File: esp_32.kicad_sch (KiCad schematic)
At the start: 20 parts, among them J1 USB_B_Micro, J2 Conn_01x22_Pin, U1 ESP32-S3-MINI-1, U2 D3V3XA4B10LP, U3 TLV75801PDRV, U4 ENS210

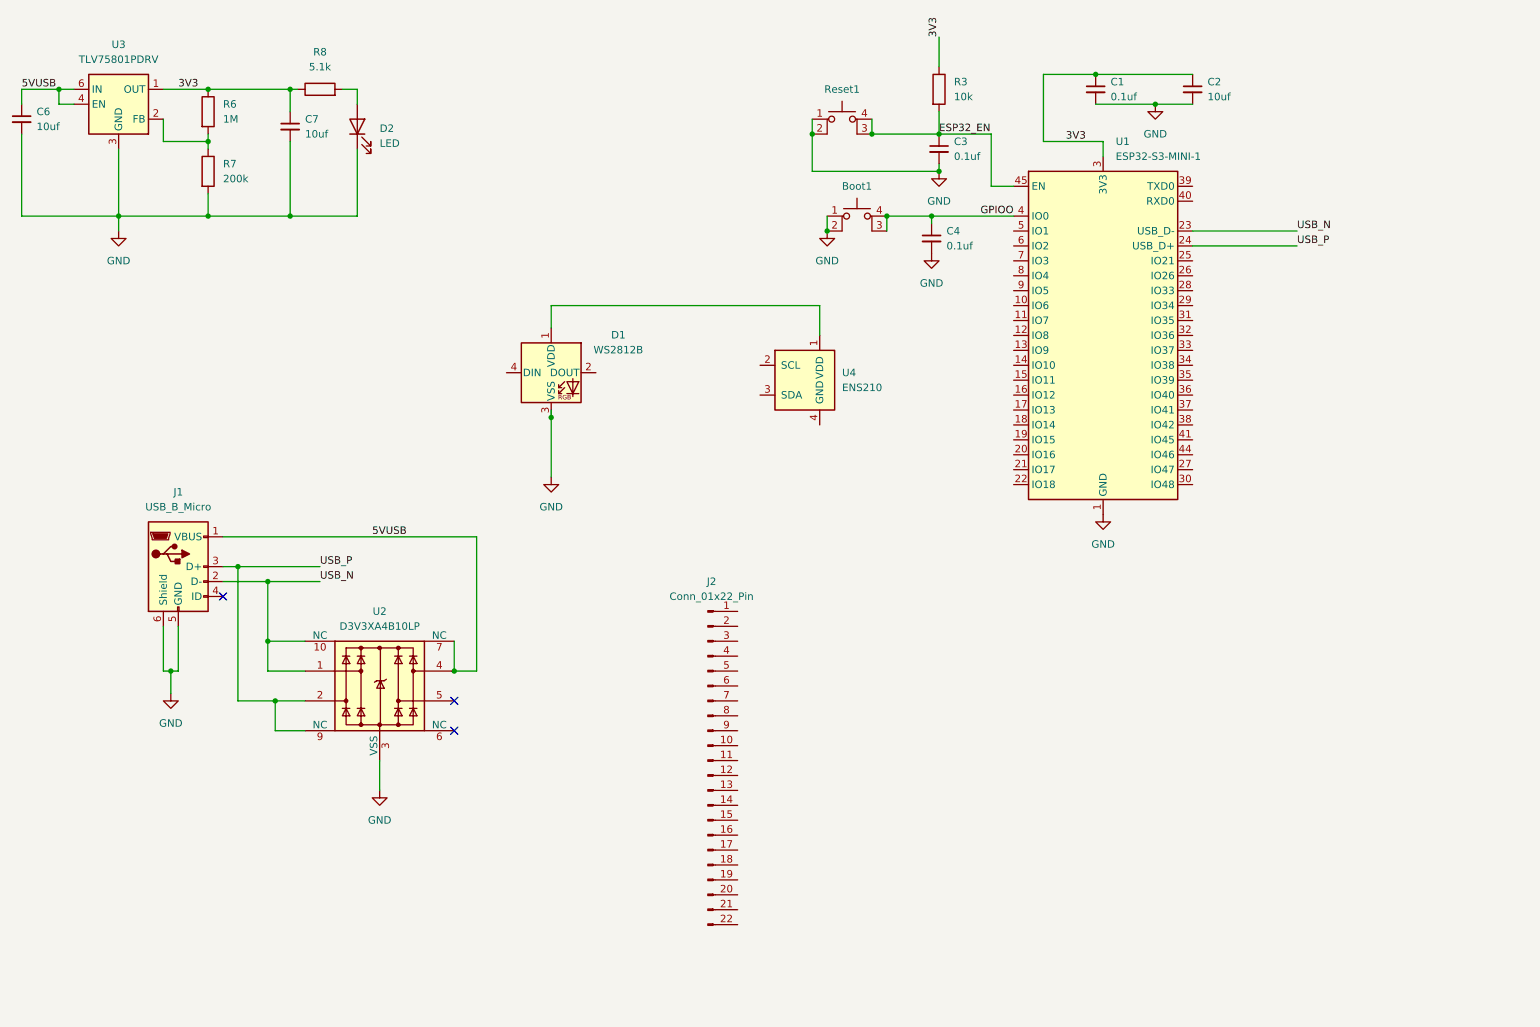
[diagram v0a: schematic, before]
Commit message: schematic
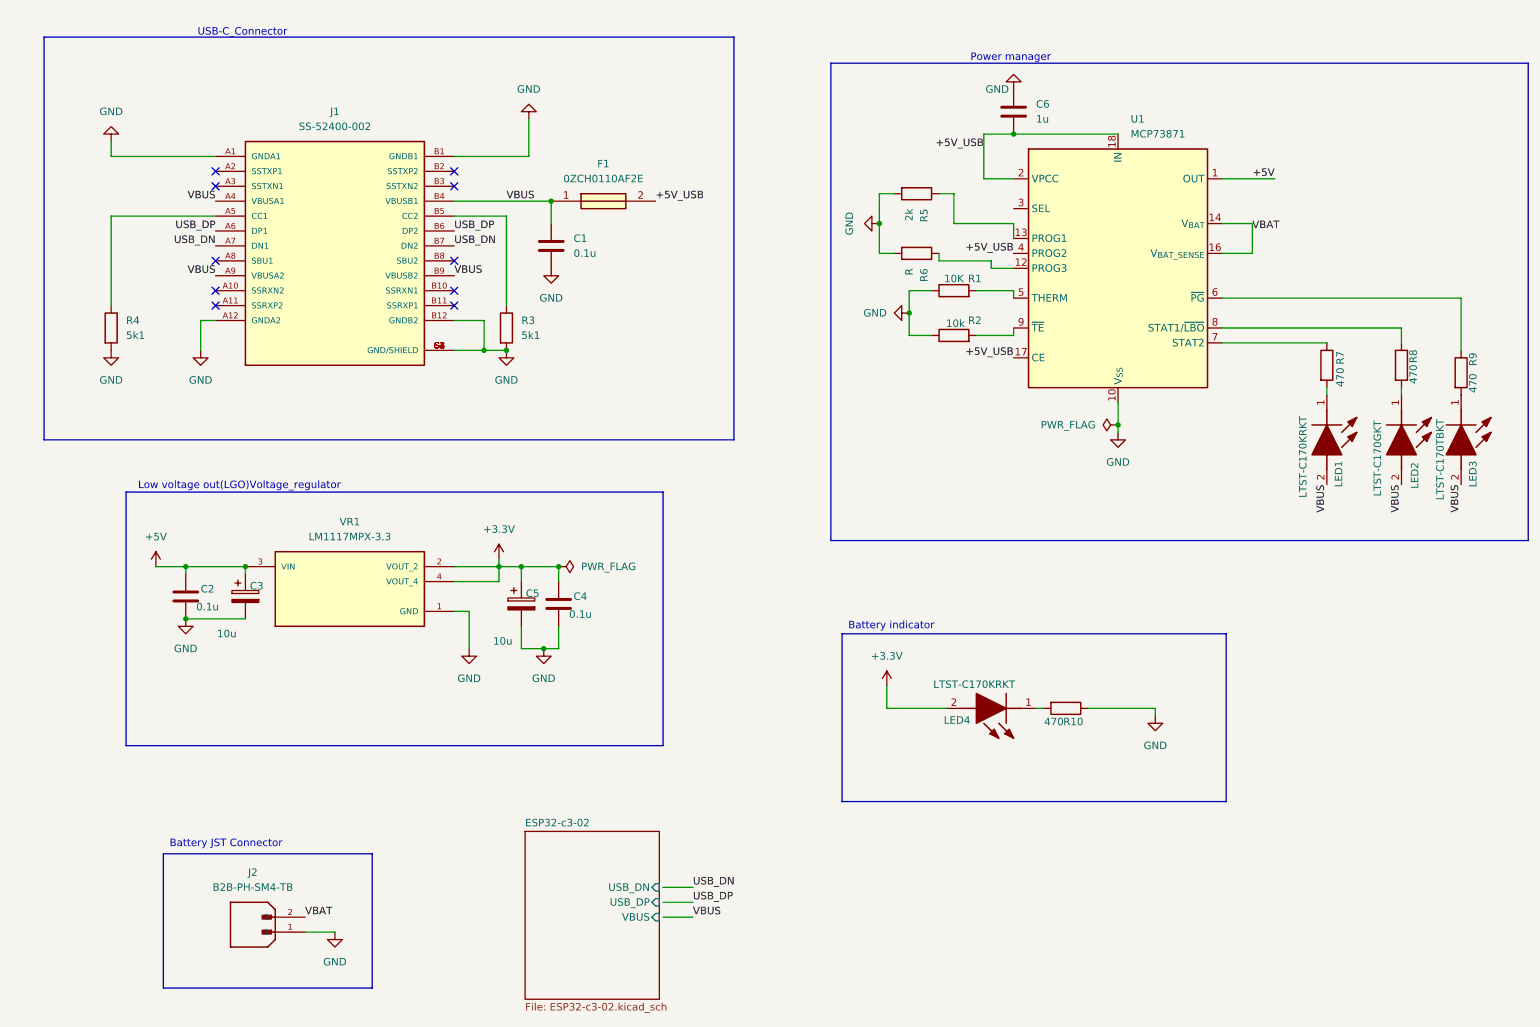
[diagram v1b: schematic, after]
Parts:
- removed Boot1, Reset1: SW_MEC_5E, Button_Switch_SMD:SW_DIP_SPSTx02_Slide_6.7x6.64mm_W6.73mm_P2.54mm_LowProfile_JPin, symbol Switch:SW_MEC_5E
- removed C1, C4: 0.1uf, Capacitor_SMD:C_0603_1608Metric, symbol Device:C_Small
- removed C2, C6, C7: 10uf, Capacitor_SMD:C_0603_1608Metric, symbol Device:C_Small
- removed C3: 0.1uf, Connector_Samtec_HPM_THT:Samtec_HPM-08-01-x-S_Straight_1x08_Pitch5.08mm, symbol Device:C_Small
- removed D1: WS2812B, LED_SMD:LED_WS2812B_PLCC4_5.0x5.0mm_P3.2mm, symbol LED:WS2812B
- removed D2: LED, LED_SMD:LED_0603_1608Metric, symbol Device:LED
- removed J1: USB_B_Micro, Connector_USB:USB_Micro-B_Molex-105017-0001, symbol Connector:USB_B_Micro
- removed J2: Conn_01x22_Pin, Connector_PinSocket_1.27mm:PinSocket_1x22_P1.27mm_Vertical, symbol Connector:Conn_01x22_Pin
- removed U1: ESP32-S3-MINI-1, RF_Module:ESP32-S2-MINI-1, symbol RF_Module:ESP32-S3-MINI-1
- removed U2: D3V3XA4B10LP, Package_DFN_QFN:Diodes_UDFN-10_1.0x2.5mm_P0.5mm, symbol Power_Protection:D3V3XA4B10LP
- removed U3: TLV75801PDRV, Package_SON:WSON-6-1EP_2x2mm_P0.65mm_EP1x1.6mm, symbol Regulator_Linear:TLV75801PDRV
- removed U4: ENS210, Package_DFN_QFN:AMS_QFN-4-1EP_2x2mm_P0.95mm_EP0.7x1.6mm, symbol Sensor_Humidity:ENS210
- added C1, C2, C4: 0.1u, symbol Device:C
- added C3, C5: 10u, symbol Device:C_Polarized
- added C6: 1u, symbol Device:C
- added F1: 0ZCH0110AF2E, FUSC3226X100N, symbol 0ZCH0110AF2E:0ZCH0110AF2E
- added J1: SS-52400-002, SS-52400-002:BELFUSE_SS-52400-002, symbol SS-52400-002:SS-52400-002
- added J2: B2B-PH-SM4-TB, B2B-PH-SM4-TB:JST_B2B-PH-SM4-TB, symbol B2B-PH-SM4-TB:B2B-PH-SM4-TB
- added LED1, LED4: LTST-C170KRKT, LEDC2012X120N, symbol LTST-C170KRKT:LTST-C170KRKT
- added LED2: LTST-C170GKT, LEDC2012X120N, symbol LTST-C170GKT:LTST-C170GKT
- added LED3: LTST-C170TBKT, LEDC2012X120N, symbol LTST-C170TBKT:LTST-C170TBKT
- added R1: 10K, symbol Device:R
- added R10, R9: 470, symbol Device:R
- added R2: 10k, symbol Device:R
- added R4: 5k1, symbol Device:R
- added R5: 2k, symbol Device:R
- added U1: MCP73871, Package_DFN_QFN:QFN-20-1EP_4x4mm_P0.5mm_EP2.5x2.5mm, symbol Battery_Management:MCP73871
- added VR1: LM1117MPX-3.3, LM1117MPX-3.3:VREG_LM1117MPX-3.3, symbol LM1117MPX-3.3:LM1117MPX-3.3
- R3: value 10k -> 5k1; footprint Resistor_SMD:R_0603_1608Metric -> (none)
- R6: value 1M -> R; footprint Resistor_SMD:R_0603_1608Metric -> (none)
- R7: value 200k -> 470; footprint Resistor_SMD:R_0603_1608Metric -> (none)
- R8: value 5.1k -> 470; footprint Resistor_SMD:R_0603_1608Metric -> (none)
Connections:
- net ESP32_EN is gone; now on net GND: R3.2
- net GND: now also R6.2, C1.2, C2.2, C3.2, C4.2, C5.2, C6.1, J1.A1 (GNDA1), J1.A12 (GNDA2), J1.B1 (GNDB1), J1.B12 (GNDB2), J1.G1 (GND/SHIELD), J1.G2 (GND/SHIELD), J1.G3 (GND/SHIELD), J1.G4 (GND/SHIELD), J1.S1 (GND/SHIELD), J1.S2 (GND/SHIELD), J1.S3 (GND/SHIELD), J1.S4 (GND/SHIELD), J2.1, R1.1, R10.1, R2.1, R4.2, R5.2, U1.10 (V_{SS}), U1.11 (V_{SS}), U1.21 (V_{SS}), VR1.1 (GND); no longer R7.2
- net at R7.1: now also U1.7 (STAT2); no longer R6.2
- net at R8.2: now also LED2.1 (K)
- removed net 3V3: R3.1, R6.1, R8.1
- new net: R6.1, U1.12 (PROG3)
- new net: R5.1, U1.13 (PROG1)
- new net: R1.2, U1.5 (THERM)
- new net: R9.1, U1.6 (~{PG})
- new net: R8.1, U1.8 (STAT1/~{LBO})
- new net: R2.2, U1.9 (~{TE})
- new net: LED1.1 (K), R7.2
- new net: J1.A5 (CC1), R4.1
- new net: J1.B5 (CC2), R3.1
- new net: LED3.1 (K), R9.2
- new net: LED4.1 (K), R10.2
- new net +3.3V: C4.1, C5.1, LED4.2 (A), VR1.2 (VOUT_2), VR1.4 (VOUT_4)
- new net +5V: C2.1, C3.1, U1.1 (OUT), U1.20 (OUT), VR1.3 (VIN)
- new net +5V_USB: C6.2, F1.2, U1.17 (CE), U1.18 (IN), U1.19 (IN), U1.2 (VPCC), U1.4 (PROG2)
- new net USB_DN: J1.A7 (DN1), J1.B7 (DN2)
- new net USB_DP: J1.A6 (DP1), J1.B6 (DP2)
- new net VBAT: J2.2, U1.14 (V_{BAT}), U1.15 (V_{BAT}), U1.16 (V_{BAT_SENSE})
- new net VBUS: C1.1, F1.1, J1.A4 (VBUSA1), J1.A9 (VBUSA2), J1.B4 (VBUSB1), J1.B9 (VBUSB2), LED1.2 (A), LED2.2 (A), LED3.2 (A)
- no-connect marks 3 -> 10
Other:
- added sheet ESP32-c3-02 (ESP32-c3-02.kicad_sch)
- note added: "Battery JST Connector"
- note added: "Battery indicator"
- note added: "Low voltage out(LGO)Voltage_regulator"
- note added: "Power manager"
- note added: "USB-C_Connector"
